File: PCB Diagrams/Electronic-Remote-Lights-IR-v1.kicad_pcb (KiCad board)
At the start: 2 copper layers, 62.7 x 69.2 mm, 17 parts, among them J1 POWER PINS, J2 POWER USB, J3 RELAY, SW1 RESET, U1 VS1338B

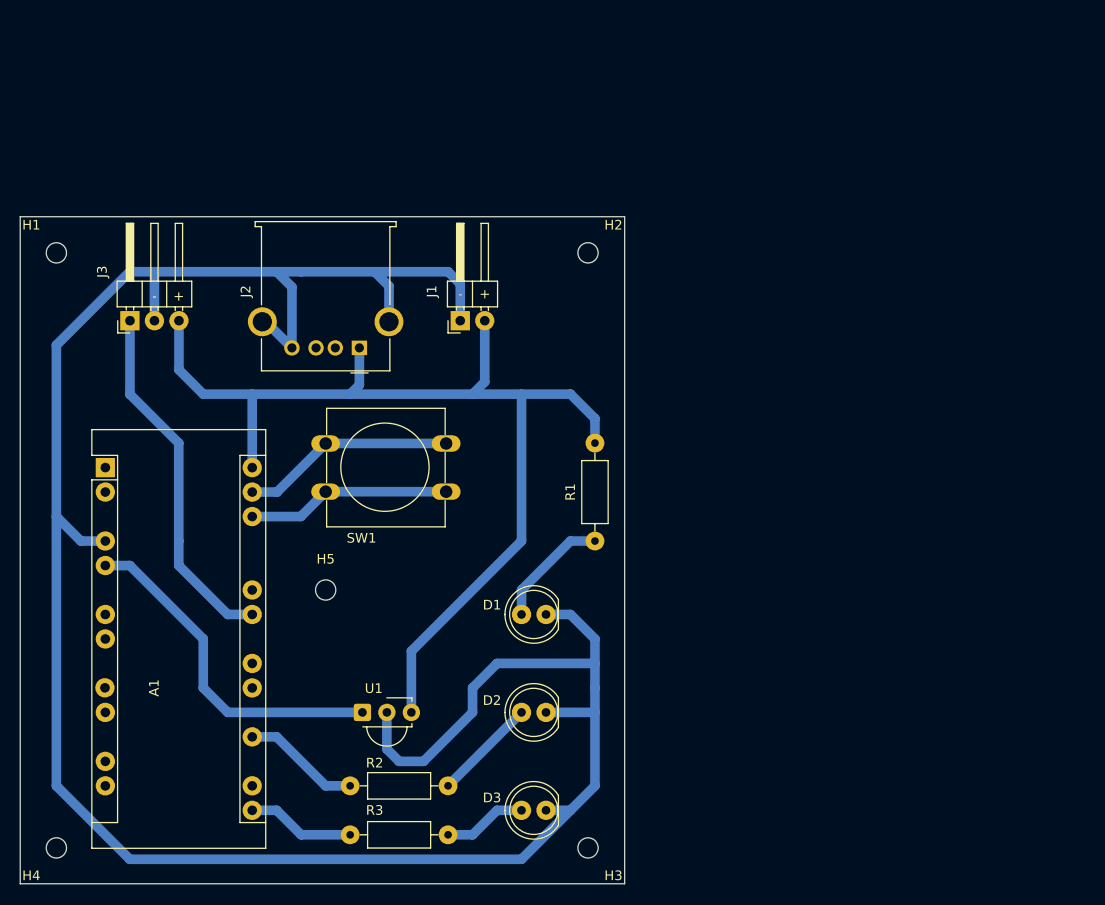
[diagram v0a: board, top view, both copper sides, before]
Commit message: update track width to 1.5mm
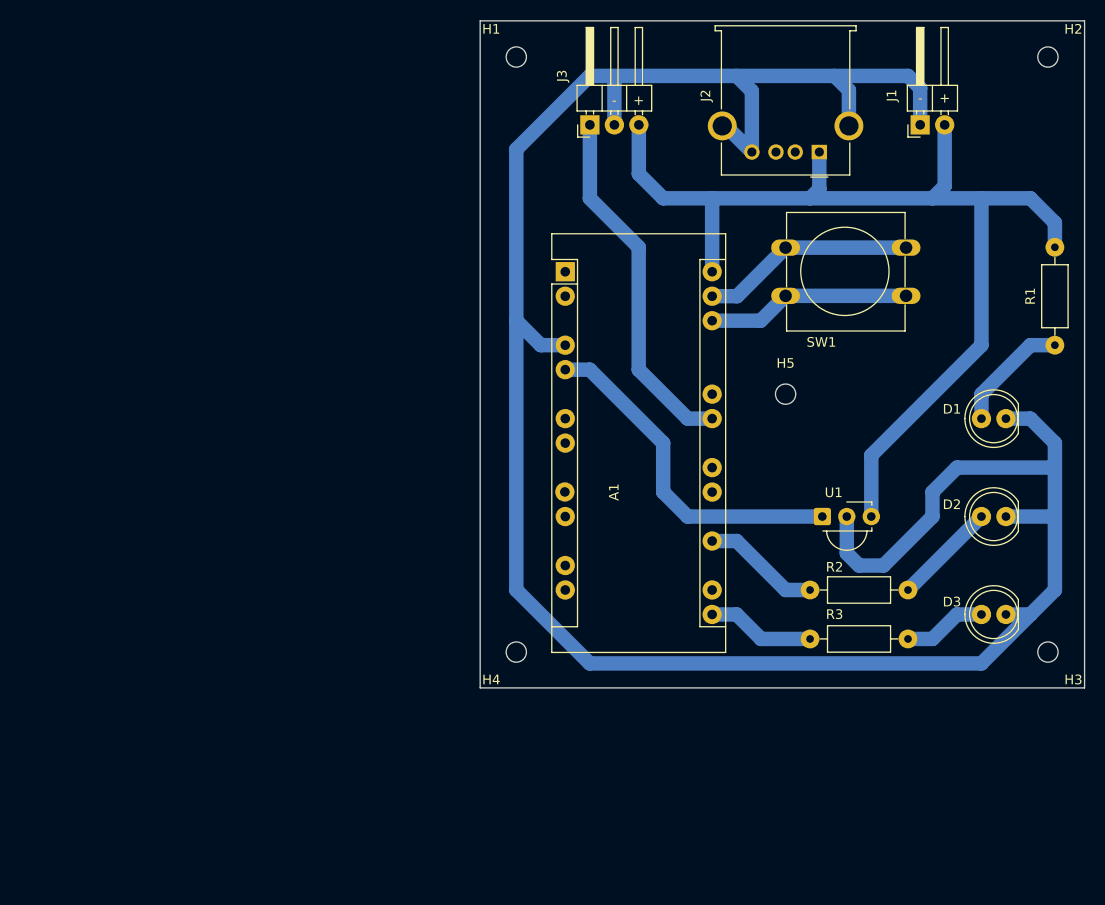
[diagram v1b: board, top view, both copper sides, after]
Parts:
- moved H5 51.9 mm to (151.9, 104.1)
- moved J2 51.9 mm to (155.4, 79.0)
- moved J3 51.9 mm to (131.6, 76.2)
- moved SW1 51.9 mm to (164.4, 93.9)
- moved A1 51.9 mm to (129.0, 91.4)
- moved H1 51.9 mm to (123.9, 69.2)
- moved H2 51.9 mm to (179.1, 69.2)
- moved R2 51.9 mm to (154.4, 124.5)
- moved R3 51.9 mm to (154.4, 129.5)
- moved D1 51.9 mm to (174.7, 106.7)
- moved D2 51.9 mm to (174.7, 116.8)
- moved D3 51.9 mm to (174.7, 127.0)
- moved H3 51.9 mm to (179.1, 130.9)
- moved H4 51.9 mm to (123.9, 130.9)
- moved R1 51.9 mm to (179.8, 88.9)
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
